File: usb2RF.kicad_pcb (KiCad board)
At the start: 4 copper layers, 40 x 15 mm, 38 parts, among them J1 USB_B_Micro, J2 SMA, J3 ARM 10Pin, U1 nRF24L01P, U2 XC6206P332MR, U3 USBLC6-2SC6, U4 STM32L432KBU6, Y1 16MHz

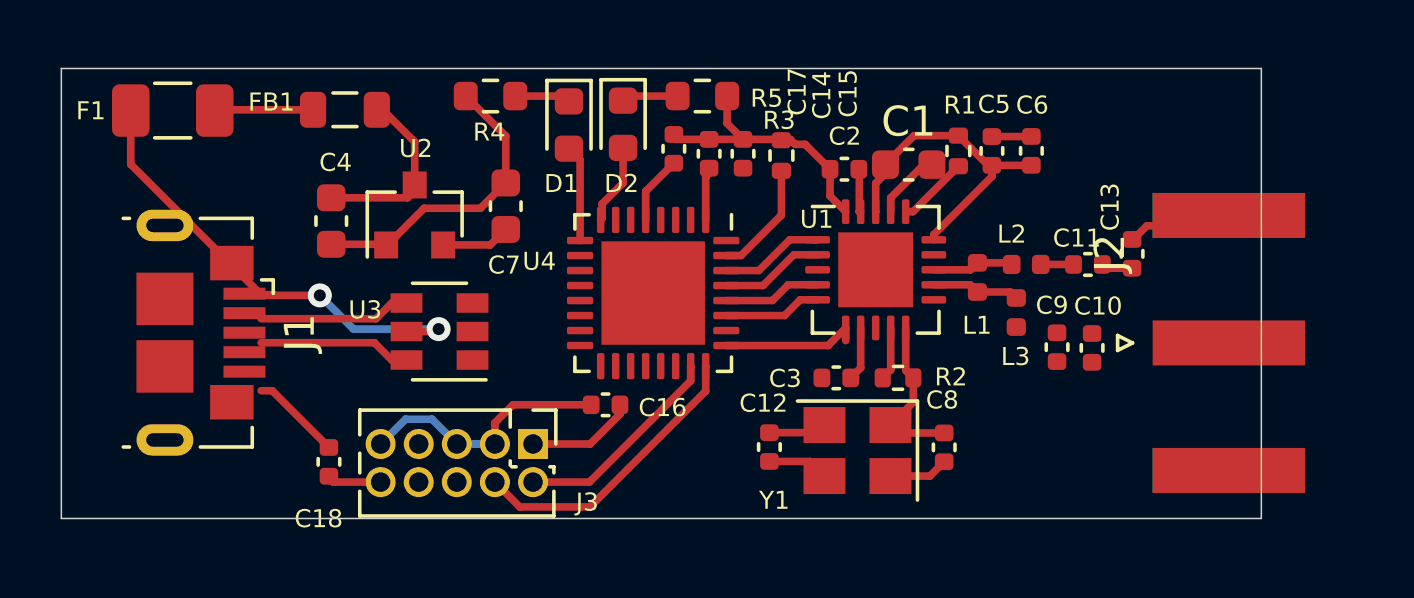
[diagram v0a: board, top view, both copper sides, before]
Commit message: [relayout]
Signed-off-by: EasonLiang <liangyx25@163.com>
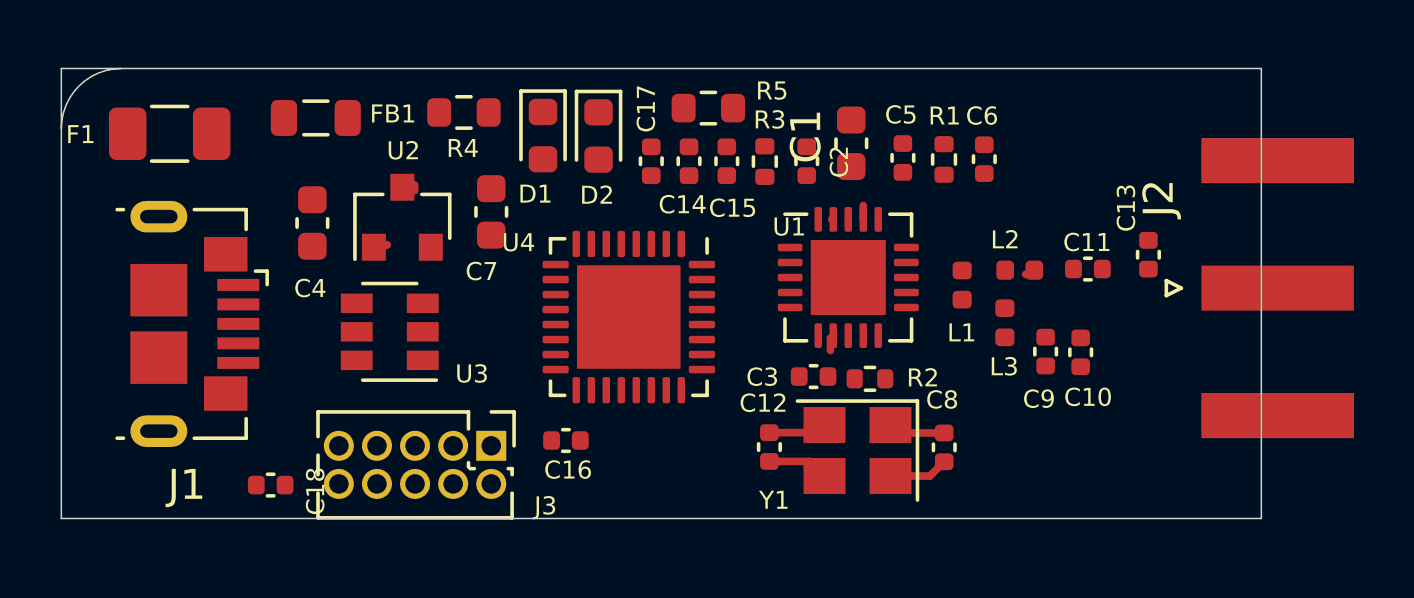
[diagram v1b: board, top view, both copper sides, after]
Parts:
- moved C5 2.98 mm to (68.1, 43.0)
- moved J2 2.45 mm to (80.5, 47.3)
- moved C18 2.09 mm to (47.0, 53.9), turned to 180 degrees
- moved C1 2.04 mm to (66.3, 42.5), turned to 90 degrees
- moved C16 1.78 mm to (56.8, 52.4)
- moved U3 1.66 mm to (50.9, 48.8)
- moved C6 1.59 mm to (70.8, 43.0)
- moved J3 1.39 mm to (54.3, 52.6)
- moved C2 1.29 mm to (64.8, 43.1), turned to 90 degrees
- moved U4 1.14 mm to (58.9, 48.3)
- moved R4 1.04 mm to (53.4, 41.5)
- moved FB1 1.01 mm to (48.5, 41.6)
- moved U1 0.95 mm to (66.2, 47.0)
- moved D1 0.94 mm to (56.1, 42.2)
- moved R2 0.94 mm to (67.0, 50.3)
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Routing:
- net GND: track 40.5 -> 4.51 mm
- net +3V3: track 22.5 -> 0.43 mm
- net +5V: track 15.9 -> 0.00 mm, vias 2 -> 0
- net SWCLK: track 9.80 -> 0.00 mm
- net SWDIO: track 7.19 -> 0.00 mm
- net Net-(C4-Pad1): track 6.21 -> 0.19 mm
- net USB_CONN_D+: track 5.09 -> 0.00 mm
- net USB_CONN_D-: track 5.06 -> 0.00 mm
- net NRF_IRQ: track 4.64 -> 0.00 mm
- net Net-(R3-Pad1): track 3.87 -> 0.00 mm
- net NRF_XC1: track 5.74 -> 1.95 mm
- net SPI3_ICS: track 3.47 -> 0.00 mm
- net NRF_CE: track 3.47 -> 0.10 mm
- net Net-(F1-Pad1): track 3.29 -> 0.00 mm
- net SPI3_MISO: track 3.26 -> 0.00 mm
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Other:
- outline, holes or cut-outs redrawn
